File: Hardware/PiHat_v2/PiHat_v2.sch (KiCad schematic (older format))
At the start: 31 parts, among them P1 RPiGPIO, P2 CONN_01X02, P3 CONN_01X08

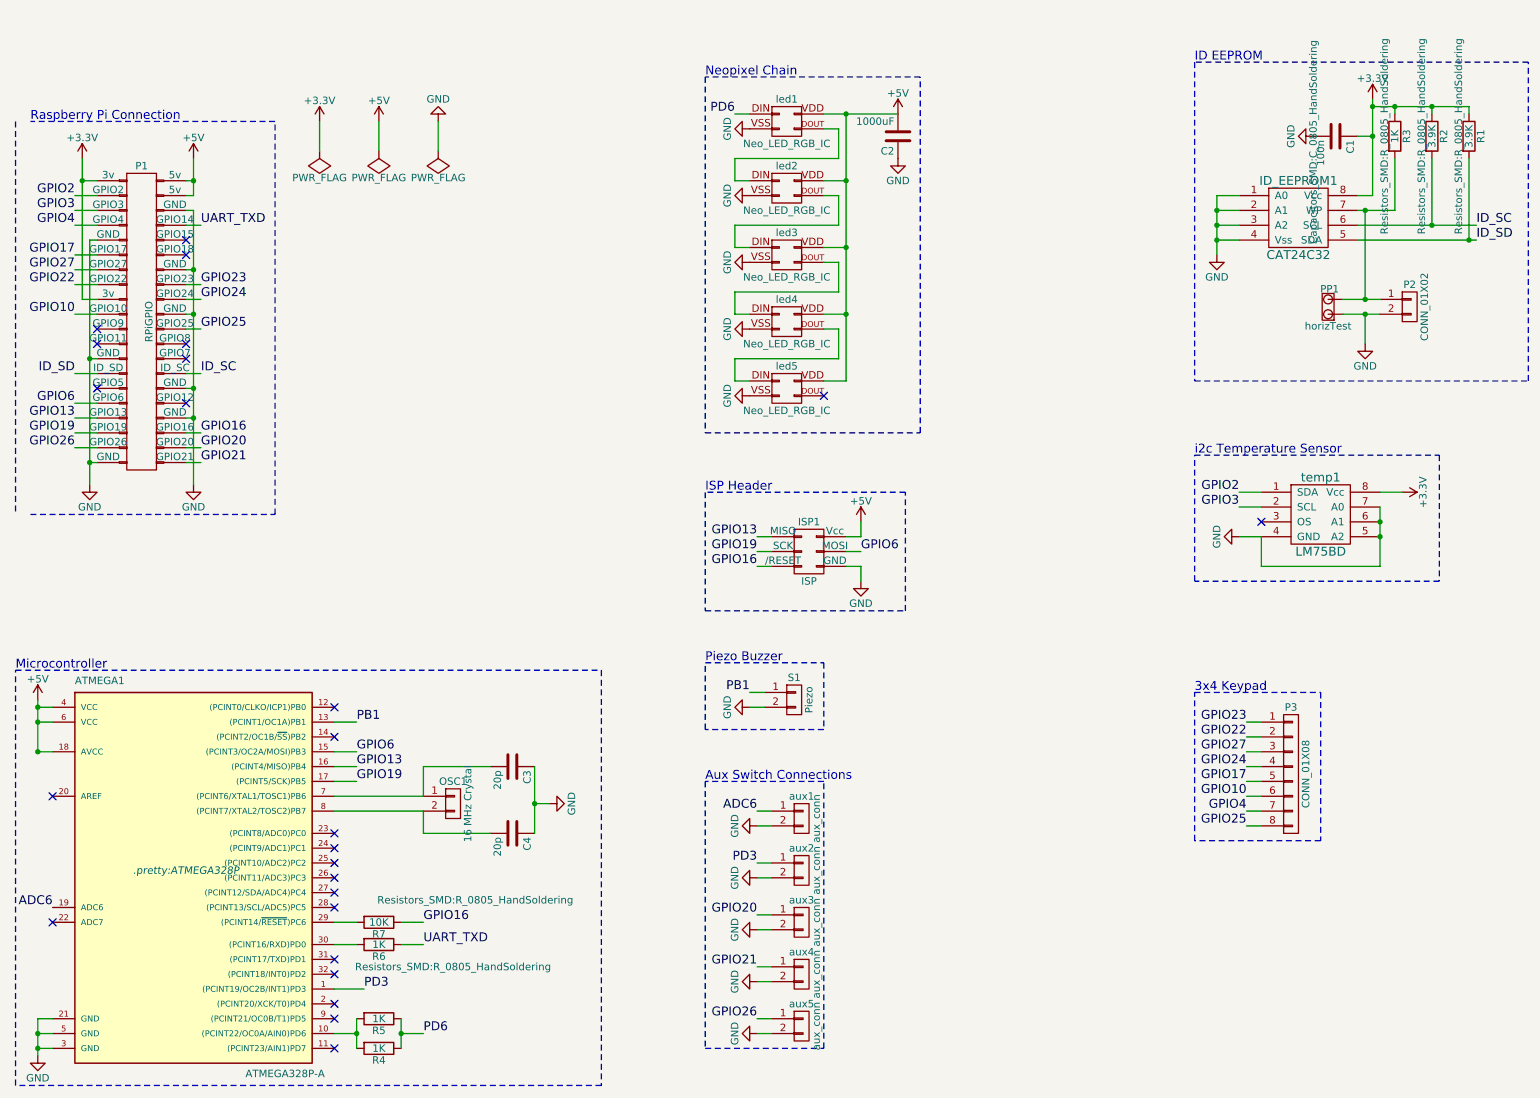
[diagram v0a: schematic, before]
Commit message: Adjust Schematic Styling
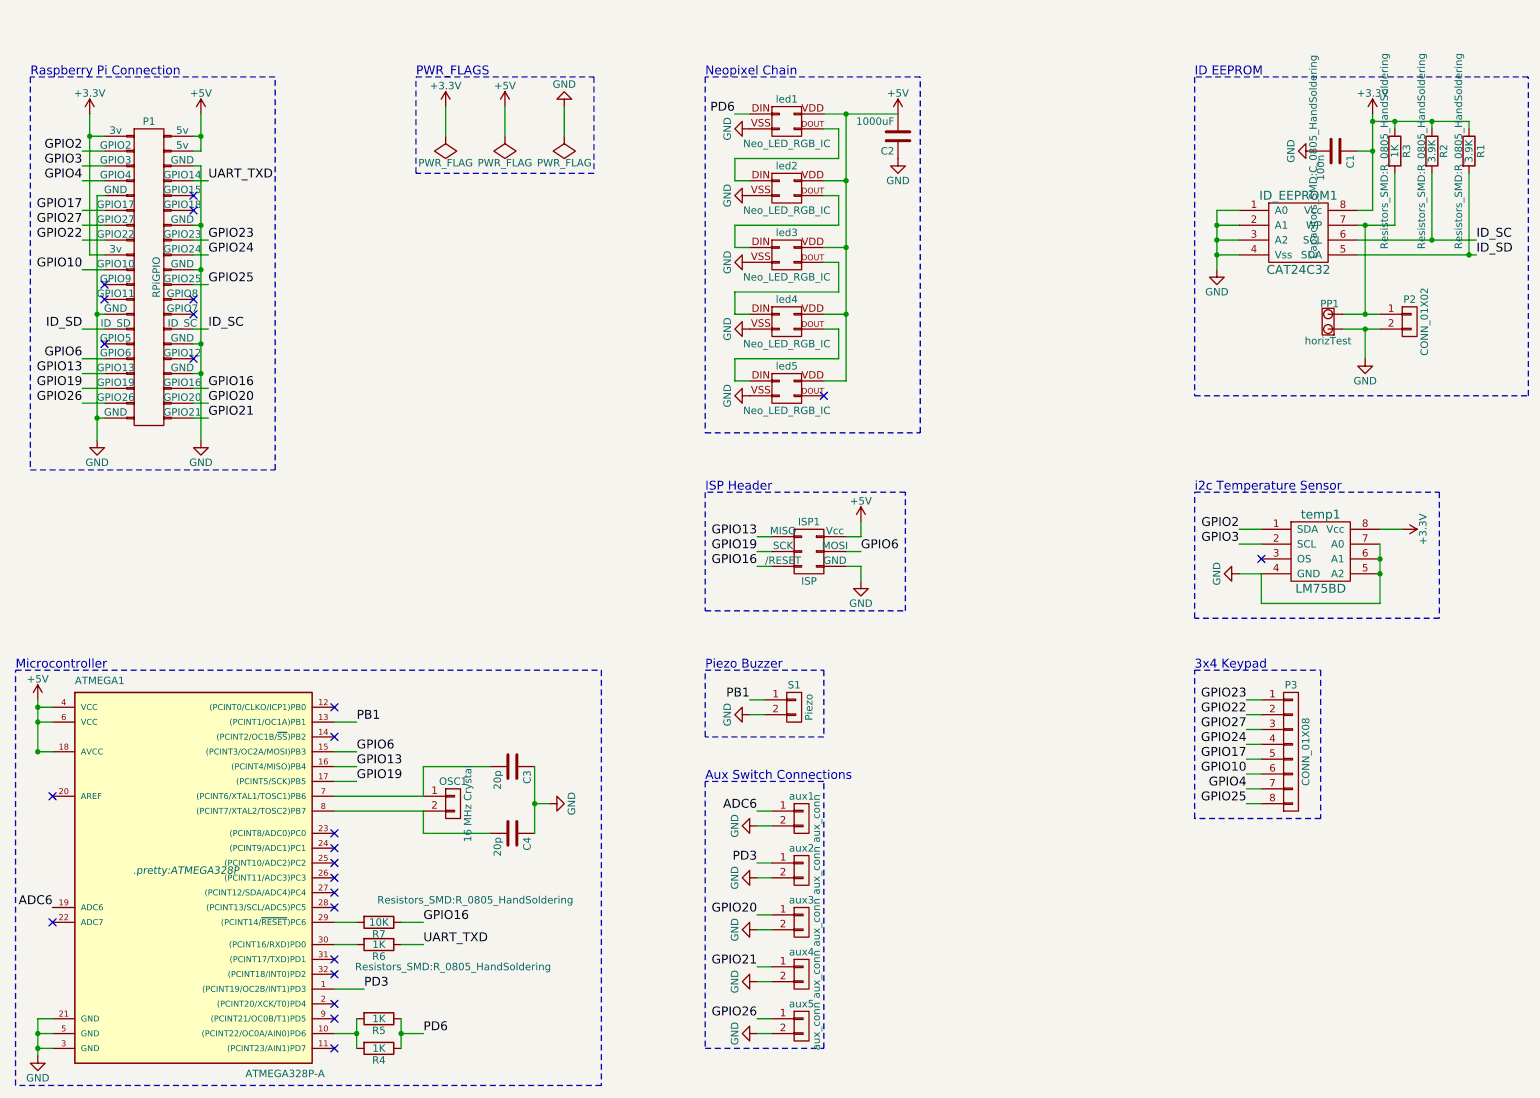
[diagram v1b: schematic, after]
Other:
- note added: "PWR_FLAGS"
- moved on the sheet: C1, ID_EEPROM1, P1, P2, P3, PP1, R1, R2, R3, S1, temp1

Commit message: Update Footprints
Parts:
- C3, C4: footprint Capacitors_THT:C_Disc_D5.0mm_W2.5mm_P2.50mm -> Capacitors_SMD:C_0603_HandSoldering
- ISP1: footprint (none) -> Pin_Headers:Pin_Header_Straight_2x03_Pitch2.54mm
- OSC1: footprint Crystals:Resonator-2pin_w10.0mm_h5.0mm -> Crystals:Crystal_SMD_HC49-SD_HandSoldering
- P1: footprint (none) -> Pin_Headers:Pin_Header_Straight_2x20_Pitch1.27mm
- R4, R5: footprint (none) -> Resistors_SMD:R_0805_HandSoldering
- aux1, aux2, aux3, aux4, aux5: footprint (none) -> Pin_Headers:Pin_Header_Straight_1x02_Pitch2.54mm
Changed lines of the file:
@@
 F 0 "OSC1" H 3700 5900 50  0000 C CNN
 F 1 "16 MHz Crystal" V 3800 5750 50  0000 C CNN
-F 2 "Crystals:Resonator-2pin_w10.0mm_h5.0mm" H 3700 5750 50  0001 C CNN
+F 2 "Crystals:Crystal_SMD_HC49-SD_HandSoldering" H 3700 5750 50  0001 C CNN
 F 3 "" H 3700 5750 50  0000 C CNN
 	1    3700 5750
@@
 F 0 "C3" H 4125 5600 50  0000 L CNN
 F 1 "20p" H 4125 5400 50  0000 L CNN
-F 2 "Capacitors_THT:C_Disc_D5.0mm_W2.5mm_P2.50mm" H 4138 5350 50  0001 C CNN
+F 2 "Capacitors_SMD:C_0603_HandSoldering" H 4138 5350 50  0001 C CNN
 F 3 "" H 4100 5500 50  0000 C CNN
 	1    4100 5500
@@
 F 0 "C4" H 4125 6050 50  0000 L CNN
 F 1 "20p" H 4125 5850 50  0000 L CNN
-F 2 "Capacitors_THT:C_Disc_D5.0mm_W2.5mm_P2.50mm" H 4138 5800 50  0001 C CNN
+F 2 "Capacitors_SMD:C_0603_HandSoldering" H 4138 5800 50  0001 C CNN
 F 3 "" H 4100 5950 50  0000 C CNN
 	1    4100 5950
@@
 F 0 "R5" V 3280 7200 50  0000 C CNN
 F 1 "1K" V 3200 7200 50  0000 C CNN
-F 2 "" V 3130 7200 50  0000 C CNN
+F 2 "Resistors_SMD:R_0805_HandSoldering" V 3130 7200 50  0001 C CNN
 F 3 "" H 3200 7200 50  0000 C CNN
 	1    3200 7200
@@
 F 0 "R4" V 3280 7400 50  0000 C CNN
 F 1 "1K" V 3200 7400 50  0000 C CNN
-F 2 "" V 3130 7400 50  0000 C CNN
+F 2 "Resistors_SMD:R_0805_HandSoldering" V 3130 7400 50  0001 C CNN
 F 3 "" H 3200 7400 50  0000 C CNN
 	1    3200 7400
@@
 F 0 "ISP1" H 6100 4250 50  0000 C CNN
 F 1 "ISP" H 6100 3850 50  0000 C CNN
-F 2 "" H 6100 2850 50  0000 C CNN
+F 2 "Pin_Headers:Pin_Header_Straight_2x03_Pitch2.54mm" H 6100 2850 50  0001 C CNN
 F 3 "" H 6100 2850 50  0000 C CNN
 	1    6100 4050
@@
 F 0 "aux1" H 6050 6000 50  0000 C CNN
 F 1 "aux_conn" V 6150 5850 50  0000 C CNN
-F 2 "" H 6050 5850 50  0000 C CNN
+F 2 "Pin_Headers:Pin_Header_Straight_1x02_Pitch2.54mm" H 6050 5850 50  0001 C CNN
 F 3 "" H 6050 5850 50  0000 C CNN
 	1    6050 5850
@@
 F 0 "aux2" H 6050 6350 50  0000 C CNN
 F 1 "aux_conn" V 6150 6200 50  0000 C CNN
-F 2 "" H 6050 6200 50  0000 C CNN
+F 2 "Pin_Headers:Pin_Header_Straight_1x02_Pitch2.54mm" H 6050 6200 50  0001 C CNN
 F 3 "" H 6050 6200 50  0000 C CNN
 	1    6050 6200
@@
 F 0 "aux3" H 6050 6700 50  0000 C CNN
 F 1 "aux_conn" V 6150 6550 50  0000 C CNN
-F 2 "" H 6050 6550 50  0000 C CNN
+F 2 "Pin_Headers:Pin_Header_Straight_1x02_Pitch2.54mm" H 6050 6550 50  0001 C CNN
 F 3 "" H 6050 6550 50  0000 C CNN
 	1    6050 6550
@@
 F 0 "aux4" H 6050 7050 50  0000 C CNN
 F 1 "aux_conn" V 6150 6900 50  0000 C CNN
-F 2 "" H 6050 6900 50  0000 C CNN
+F 2 "Pin_Headers:Pin_Header_Straight_1x02_Pitch2.54mm" H 6050 6900 50  0001 C CNN
 F 3 "" H 6050 6900 50  0000 C CNN
 	1    6050 6900
@@
 F 0 "aux5" H 6050 7400 50  0000 C CNN
 F 1 "aux_conn" V 6150 7250 50  0000 C CNN
-F 2 "" H 6050 7250 50  0000 C CNN
+F 2 "Pin_Headers:Pin_Header_Straight_1x02_Pitch2.54mm" H 6050 7250 50  0001 C CNN
 F 3 "" H 6050 7250 50  0000 C CNN
 	1    6050 7250
@@
 F 0 "P1" H 1650 3250 50  0000 C CNN
 F 1 "RPiGPIO" V 1700 2200 50  0000 C CNN
-F 2 "" H 1700 1250 50  0000 C CNN
+F 2 "Pin_Headers:Pin_Header_Straight_2x20_Pitch1.27mm" H 1700 1250 50  0001 C CNN
 F 3 "" H 1700 1250 50  0000 C CNN
 	1    1650 2200
